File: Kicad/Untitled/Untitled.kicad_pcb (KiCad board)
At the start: 2 copper layers, 27.3 x 54.9 mm, 52 parts, among them J1 USB_C_Receptacle_USB2.0_14P, J2 Conn_01x04_Socket, J3 Screw_Terminal_01x02, J4 Conn_01x16_Pin, J5 Conn_01x04_Socket, J6 Conn_01x13_Pin, SW1 SW_Push_45deg, SW2 SW_Push_45deg, SW3 SW_Push, SW4 SW_Push, U1 NCP1117-3.3_TO252, U2 NCP1117-3.3_TO252, U3 APS6404L-3SQRx-ZR, U4 ESP32-S3, Y1 32.768kHz, Y2 40 MHz

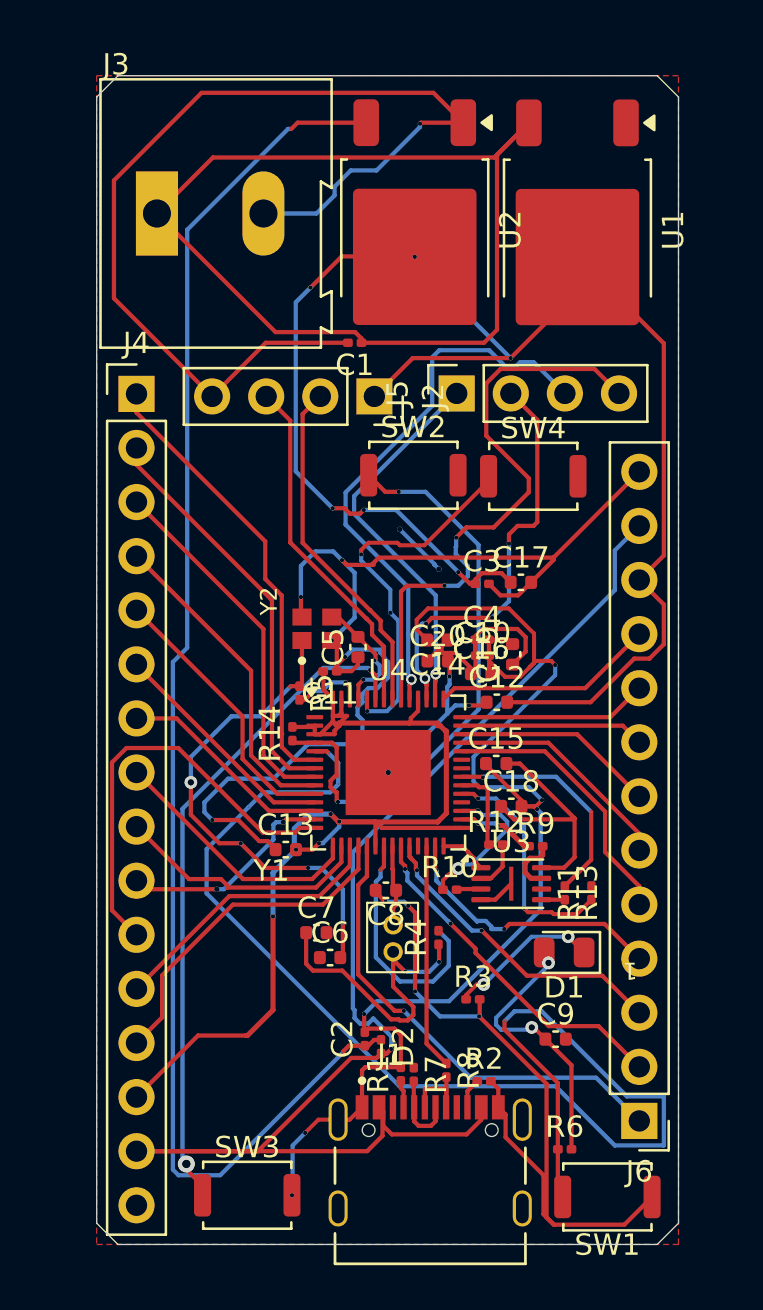
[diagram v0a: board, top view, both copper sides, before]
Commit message: pcb update
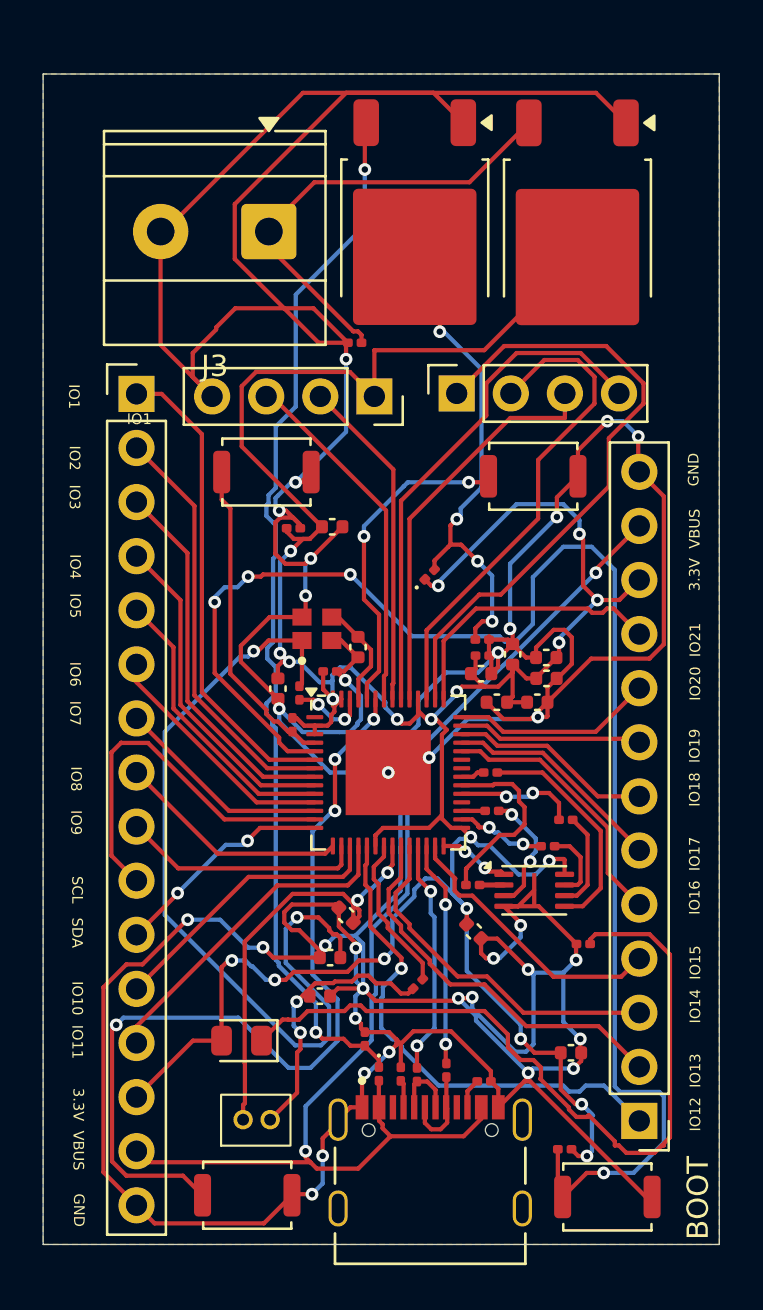
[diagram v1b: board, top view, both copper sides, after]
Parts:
- added D3: D, Diode_SMD:D_0201_0603Metric, F.Cu at (127.6, 93.3)
- added G***: LOGO, LOGO, B.Cu at (125.3, 75.6)
- added G***: LOGO, LOGO, B.Cu at (124.0, 101.3)
- J3: footprint TerminalBlock:TerminalBlock_Altech_AK300-2_P5.00mm -> TerminalBlock_Phoenix:TerminalBlock_Phoenix_MKDS-1,5-2-5.08_1x02_P5.08mm_Horizontal
- moved D1 15.7 mm to (118.8, 115.2)
- moved Y1 10.7 mm to (119.5, 118.9), turned to 90 degrees
- moved C17 9.24 mm to (123.0, 91.1)
- moved C3 9.24 mm to (121.2, 91.1)
- moved C15 7.95 mm to (129.7, 110.1), turned to 135 degrees
- moved C13 7.57 mm to (120.5, 98.7), turned to 90 degrees
- moved SW2 6.90 mm to (120.0, 88.5)
- moved R13 6.65 mm to (130.5, 102.6), turned to 0 degrees
- moved R3 5.80 mm to (134.8, 110.7), turned to 180 degrees
- moved J3 5.32 mm to (120.1, 77.2), turned to 180 degrees
- moved C20 5.18 mm to (133.1, 98.2)
- moved C14 5.18 mm to (133.1, 97.2)
- moved C18 5.04 mm to (132.7, 99.3)
- moved R10 4.20 mm to (130.6, 104.4)
- moved R11 3.63 mm to (134.0, 104.8), turned to 0 degrees
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- renumbered SW1 to BOOT
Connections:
- C4 pad 1: +3V3 -> Net-(D3-A)
- U2 pad 2: +3V3 -> Net-(D3-A)
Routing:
- net GND: track 212.9 -> 311.6 mm, vias 19 -> 34
- net Net-(D1-K): track 7.18 -> 37.1 mm, vias 2 -> 0
- net Net-(J3-Pin_1): track 48.4 -> 21.6 mm
- net Net-(D3-A): track 0.00 -> 23.2 mm, vias 0 -> 4
- net Net-(D2-K): track 67.4 -> 50.3 mm
- net Net-(C6-Pad2): track 23.2 -> 39.7 mm, vias 5 -> 2
- net XTAL_32K_N: track 3.83 -> 20.2 mm, vias 0 -> 2
- net +3V3: track 165.3 -> 150.0 mm, vias 13 -> 20
- net Net-(U4-CHIP_PU): track 27.8 -> 15.1 mm, vias 2 -> 0
- net MTCK: track 17.9 -> 29.9 mm, vias 1 -> 0
- net Net-(U4-GPIO0): track 59.6 -> 71.1 mm
- net Net-(U4-GPIO19/USB_D-): track 0.00 -> 11.1 mm, vias 0 -> 2
- net Net-(U4-GPIO45): track 31.6 -> 41.4 mm, vias 2 -> 4
- net Net-(U4-SPID): track 10.8 -> 1.11 mm, vias 2 -> 0
- net SPID: track 1.09 -> 10.7 mm
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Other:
- board size 27.3 x 54.9 mm -> 31.8 x 55 mm
- board text added: "3.3V VBUS"
- board text added: "GND"
- board text added: "IO1"
- board text added: "IO10 IO11"
- board text added: "IO12 IO13"
- board text added: "IO14 IO15"
- board text added: "IO16 IO17"
- board text added: "IO18 IO19"
- board text added: "IO2 IO3"
- board text added: "IO20 IO21"
- board text added: "IO4 IO5"
- board text added: "IO6 IO7"
- board text added: "IO8 IO9"
- board text added: "SAMHITHS ESP32-S3 SOC BOARD"
- board text added: "SCL SDA"

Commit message: journal update, pcb update
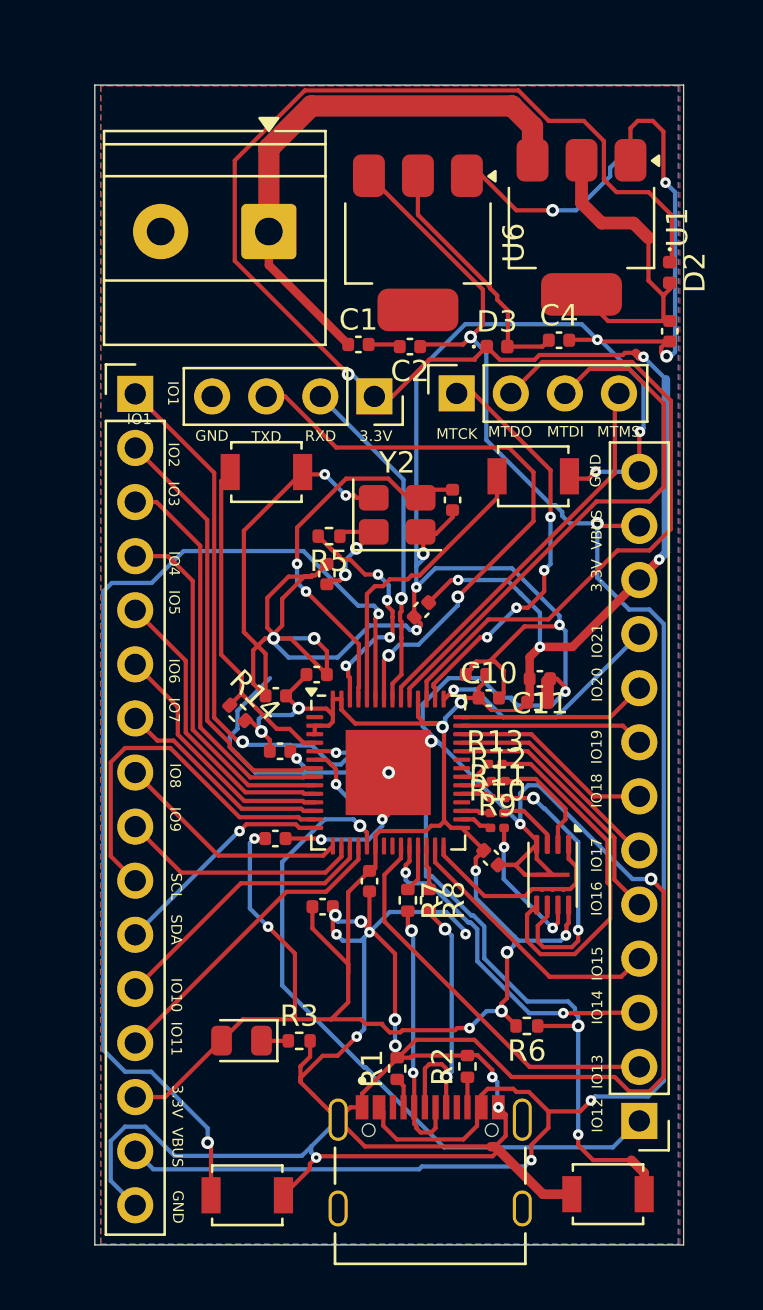
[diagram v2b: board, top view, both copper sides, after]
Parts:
- removed BOOT: SW_Push_45deg, Button_Switch_SMD:SW_Push_SPST_NO_Alps_SKRK
- removed C7, C8: 12pF, Capacitor_SMD:C_0402_1005Metric
- removed R4: 200, Resistor_SMD:R_0201_0603Metric
- removed U2: NCP1117-3.3_TO252, Package_TO_SOT_SMD:TO-252-2
- removed Y1: 32.768kHz, AB38T_32_768KHZ:XTAL_AB38T-32.768KHZ
- added SW1: SW_Push_45deg, Button_Switch_SMD:SW_SPST_B3U-1000P, F.Cu at (136.0, 122.4)
- added U6: LD1117S33TR_SOT223, Package_TO_SOT_SMD:SOT-223-3_TabPin2, F.Cu at (127.1, 77.7)
- C1, C10, C11, C2, C3, C4: footprint Capacitor_SMD:C_0201_0603Metric -> Capacitor_SMD:C_0402_1005Metric
- D2, D3: footprint Diode_SMD:D_0201_0603Metric -> Diode_SMD:D_0402_1005Metric
- R1, R14, R2, R3, R5, R6, R7, R8: footprint Resistor_SMD:R_0201_0603Metric -> Resistor_SMD:R_0402_1005Metric
- SW2, SW3, SW4: footprint Button_Switch_SMD:SW_Push_SPST_NO_Alps_SKRK -> Button_Switch_SMD:SW_SPST_B3U-1000P
- U1: footprint Package_TO_SOT_SMD:TO-252-2 -> Package_TO_SOT_SMD:SOT-223-3_TabPin2
- Y2: footprint CX2016DB40000D0FLJCC:OSC_CX2016DB40000D0FLJCC -> Crystal:Crystal_SMD_SeikoEpson_FA238-4Pin_3.2x2.5mm
- moved D2 40.0 mm to (138.9, 79.1)
- moved C2 32.6 mm to (126.7, 82.6), turned to 180 degrees
- moved C3 19.9 mm to (138.9, 81.9), turned to -90 degrees
- moved C6 18.0 mm to (122.8, 93.3), turned to -90 degrees
- moved C19 14.8 mm to (122.6, 108.9), turned to 0 degrees
- moved C20 14.8 mm to (120.4, 105.7)
- moved C4 14.5 mm to (133.7, 82.3)
- moved R3 14.1 mm to (121.5, 115.2), turned to 0 degrees
- moved C9 12.4 mm to (124.8, 107.7), turned to -90 degrees
- moved D3 11.2 mm to (130.8, 82.6), turned to 0 degrees
- moved C12 10.4 mm to (120.4, 99.0)
- moved C11 9.86 mm to (132.8, 98.2)
- moved C5 8.21 mm to (128.7, 89.8)
- moved R7 8.20 mm to (126.6, 108.6)
- moved R8 8.02 mm to (127.6, 108.6)
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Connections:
- C2 pad 1: Net-(D2-K) -> VBUS
- C3 pad 1: +3V3 -> Net-(D2-A)
- D2 pad 1: Net-(D2-K) -> +3V3
- D2 pad 2: VBUS -> Net-(D2-A)
- U1 pad 2: +3V3 -> Net-(D2-A)
- U4 pad 21: XTAL_32K_P -> unconnected-(U4-XTAL_32K_P-Pad21)
- U4 pad 22: XTAL_32K_N -> unconnected-(U4-XTAL_32K_N-Pad22)
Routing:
- net Net-(D2-K): track 50.3 -> 0.00 mm, vias 2 -> 0
- net Net-(U4-GPIO0): track 71.1 -> 34.5 mm, vias 4 -> 3
- net Net-(D1-K): track 37.1 -> 1.19 mm
- net VBUS: track 57.7 -> 93.6 mm, vias 2 -> 4
- net Net-(C6-Pad2): track 39.7 -> 5.47 mm
- net +3V3: track 150.0 -> 176.8 mm, vias 20 -> 16
- net XTAL_32K_N: track 20.2 -> 0.00 mm, vias 2 -> 0
- net Net-(D2-A): track 0.00 -> 15.3 mm
- net Net-(C7-Pad1): track 13.1 -> 0.00 mm, vias 2 -> 0
- net XIN: track 5.03 -> 18.0 mm, vias 0 -> 2
- net IO1: track 22.6 -> 34.8 mm, vias 0 -> 2
- net GND: track 311.6 -> 300.2 mm, vias 34 -> 33
- net TXD: track 16.7 -> 28.1 mm, vias 0 -> 2
- net Net-(D3-A): track 23.2 -> 11.9 mm, vias 4 -> 0
- net MTCK: track 29.9 -> 19.5 mm, vias 0 -> 4
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- added copper zone on B.Cu, net GND
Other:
- board size 31.8 x 55 mm -> 27.7 x 54.5 mm
- board text added: "3.3V"
- board text added: "MTCK"
- board text added: "MTDI"
- board text added: "MTDO"
- board text added: "MTMS"
- board text added: "RXD"
- board text added: "TXD"
